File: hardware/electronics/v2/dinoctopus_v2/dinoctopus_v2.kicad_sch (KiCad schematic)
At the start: 8 parts, among them J1 Conn_01x04_Socket, J2 Conn_01x03_Pin, J3 Conn_01x05_Pin, J4 Conn_01x05_Pin, J5 Conn_01x03_Pin, J6 Conn_01x04_Pin, J7 Conn_01x03_Pin, U1 Pico mounting

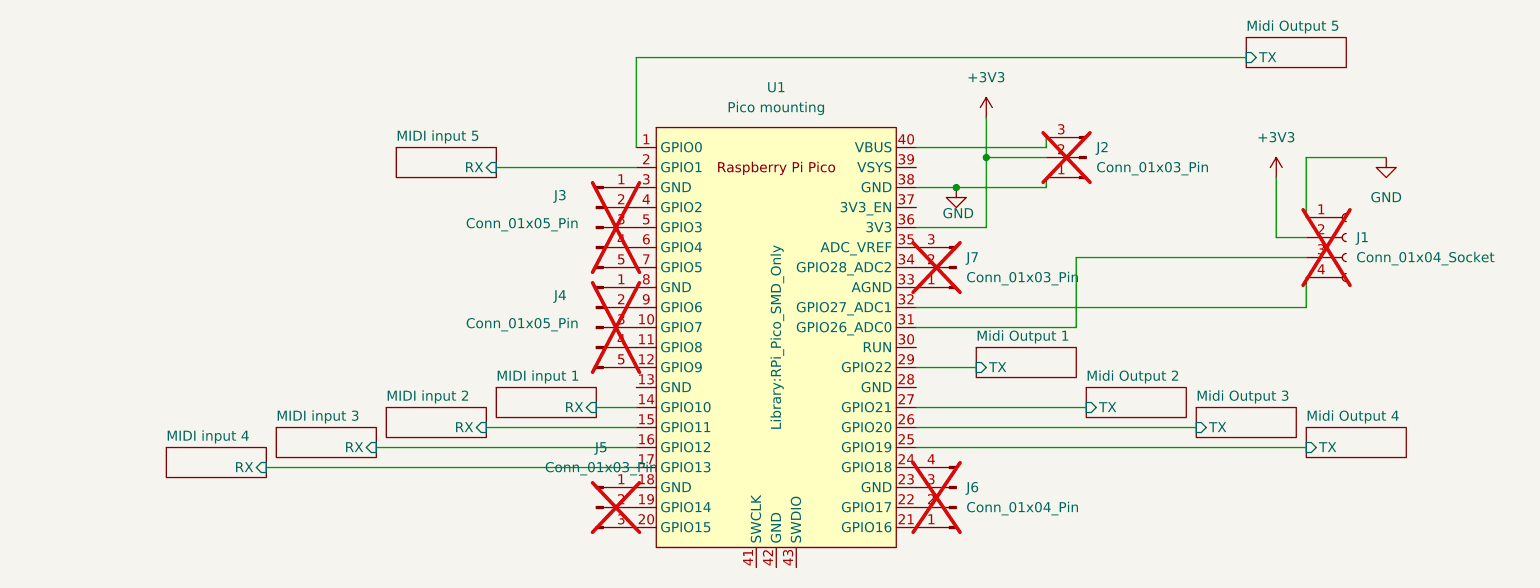
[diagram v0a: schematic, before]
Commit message: giant mess
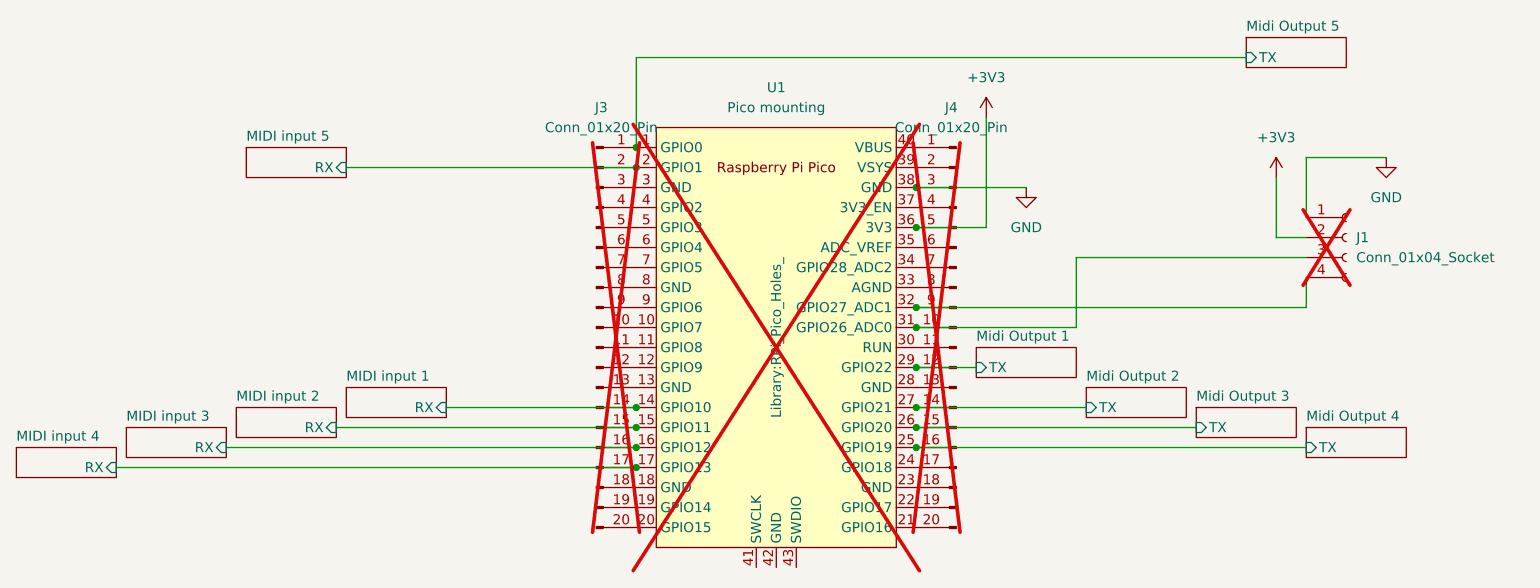
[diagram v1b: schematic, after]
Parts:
- removed J2, J5, J7: Conn_01x03_Pin, Connector_PinHeader_2.54mm:PinHeader_1x03_P2.54mm_Vertical, symbol Connector:Conn_01x03_Pin
- removed J3, J4: Conn_01x05_Pin, Connector_PinHeader_2.54mm:PinHeader_1x05_P2.54mm_Vertical, symbol Connector:Conn_01x05_Pin
- removed J6: Conn_01x04_Pin, Connector_PinHeader_2.54mm:PinHeader_1x04_P2.54mm_Vertical, symbol Connector:Conn_01x04_Pin
- added J3, J4: Conn_01x20_Pin, Connector_PinSocket_2.54mm:PinSocket_1x20_P2.54mm_Vertical, symbol Connector:Conn_01x20_Pin
- U1: footprint Library:RPi_Pico_SMD_Only -> Library:RPi_Pico_Holes_; now not fitted; now left out of the parts list
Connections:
- net +3V3: now also J4.5 (Pin_5)
- net GND: now also J4.3 (Pin_3)
- net MIDI input 1/RX: now also J3.14 (Pin_14)
- net MIDI input 2/RX: now also J3.15 (Pin_15)
- net MIDI input 3/RX: now also J3.16 (Pin_16)
- net MIDI input 4/RX: now also J3.17 (Pin_17)
- net MIDI input 5/RX: now also J3.2 (Pin_2)
- net Midi Output 1/TX: now also J4.12 (Pin_12)
- net Midi Output 2/TX: now also J4.14 (Pin_14)
- net Midi Output 3/TX: now also J4.15 (Pin_15)
- net Midi Output 4/TX: now also J4.16 (Pin_16)
- net Midi Output 5/TX: now also J3.1 (Pin_1)
- net at U1.8 (GND): now also J3.8 (Pin_8)
- net at U1.9 (GPIO6): now also J3.9 (Pin_9)
- net at U1.10 (GPIO7): now also J3.10 (Pin_10)
- net at U1.11 (GPIO8): now also J3.11 (Pin_11)
- net at U1.12 (GPIO9): now also J3.12 (Pin_12)
- net at U1.21 (GPIO16): now also J4.20 (Pin_20)
- net at U1.22 (GPIO17): now also J4.19 (Pin_19)
- net at U1.23 (GND): now also J4.18 (Pin_18)
- net at U1.24 (GPIO18): now also J4.17 (Pin_17)
- net at J1.3 (Pin_3), U1.31 (GPIO26_ADC0): now also J4.10 (Pin_10)
- net at J1.4 (Pin_4), U1.32 (GPIO27_ADC1): now also J4.9 (Pin_9)
- net at U1.33 (AGND): now also J4.8 (Pin_8)
- net at U1.34 (GPIO28_ADC2): now also J4.7 (Pin_7)
- net at U1.35 (ADC_VREF): now also J4.6 (Pin_6)
- net at U1.40 (VBUS): now also J4.1 (Pin_1)
- net at U1.3 (GND): now also J3.3 (Pin_3)
- net at U1.4 (GPIO2): now also J3.4 (Pin_4)
- net at U1.5 (GPIO3): now also J3.5 (Pin_5)
- net at U1.6 (GPIO4): now also J3.6 (Pin_6)
- net at U1.7 (GPIO5): now also J3.7 (Pin_7)
- net at U1.13 (GND): now also J3.13 (Pin_13)
- net at U1.18 (GND): now also J3.18 (Pin_18)
- net at U1.19 (GPIO14): now also J3.19 (Pin_19)
- net at U1.20 (GPIO15): now also J3.20 (Pin_20)
- net at U1.28 (GND): now also J4.13 (Pin_13)
- net at U1.30 (RUN): now also J4.11 (Pin_11)
- net at U1.37 (3V3_EN): now also J4.4 (Pin_4)
- net at U1.39 (VSYS): now also J4.2 (Pin_2)
